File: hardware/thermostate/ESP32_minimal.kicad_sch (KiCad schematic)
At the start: 28 parts, among them IC1 L8050QLT1G, IC2 L8050QLT1G, P1 USB_C_Plug_USB2.0, SW1 SW_Push, SW2 SW_Push, U1 ESP32-S3-WROOM-1, U2 LM1117-3.3

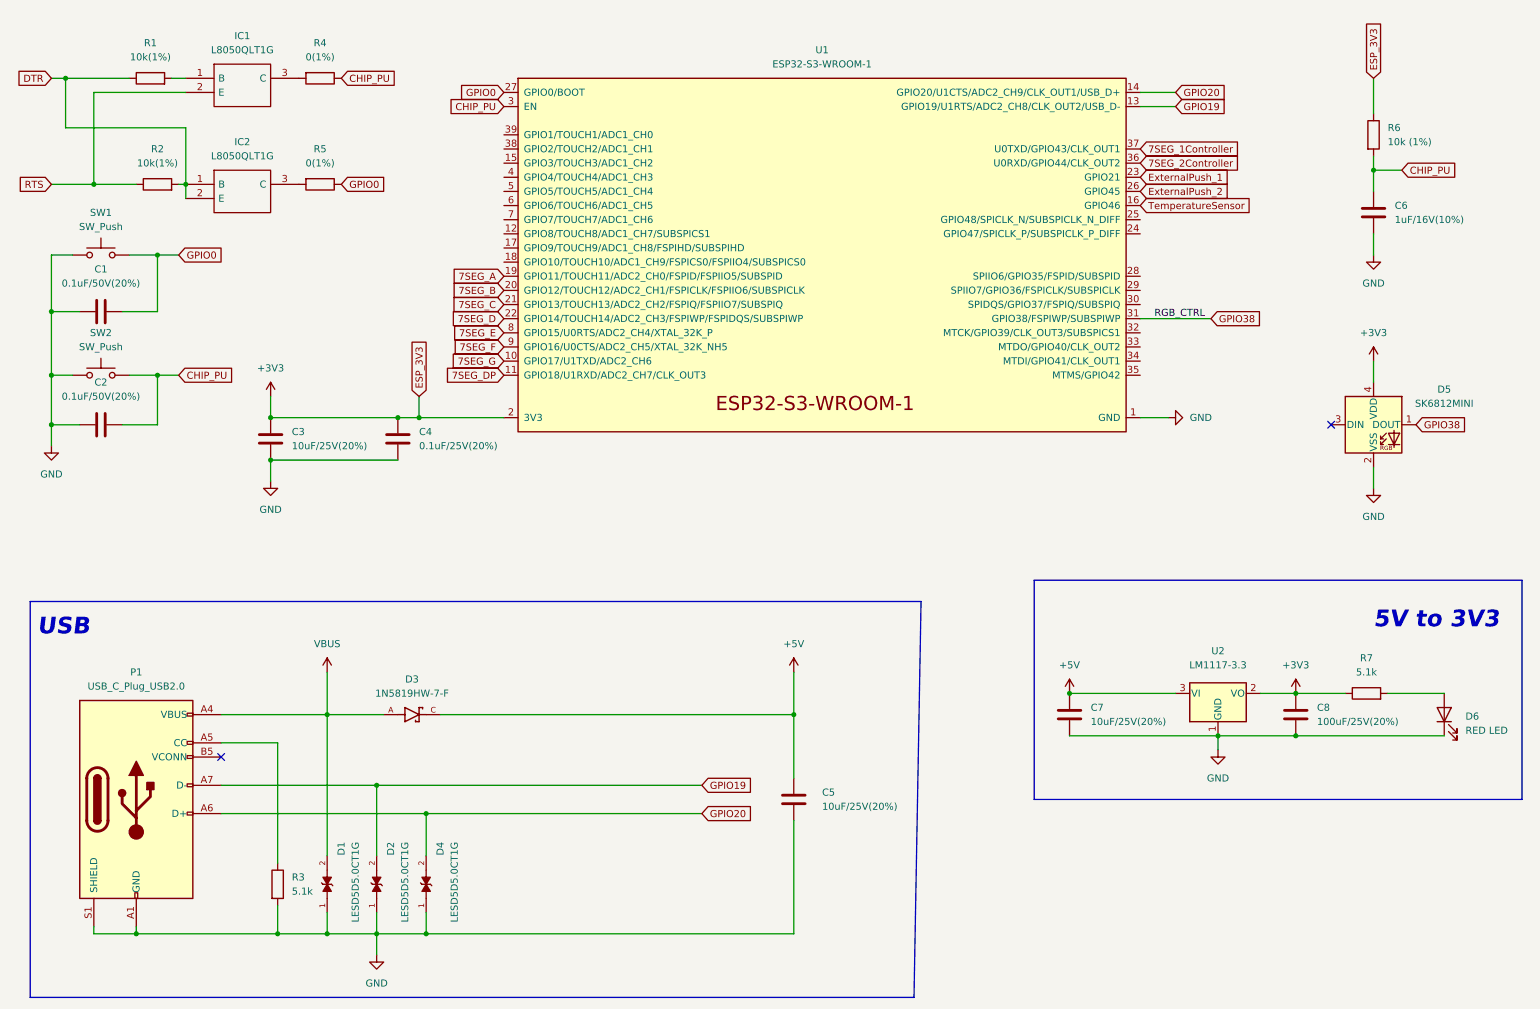
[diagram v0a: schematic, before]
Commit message: Start desing PCB
Signed-off-by: Javier <javierfernandezvillasante@gmail.com>
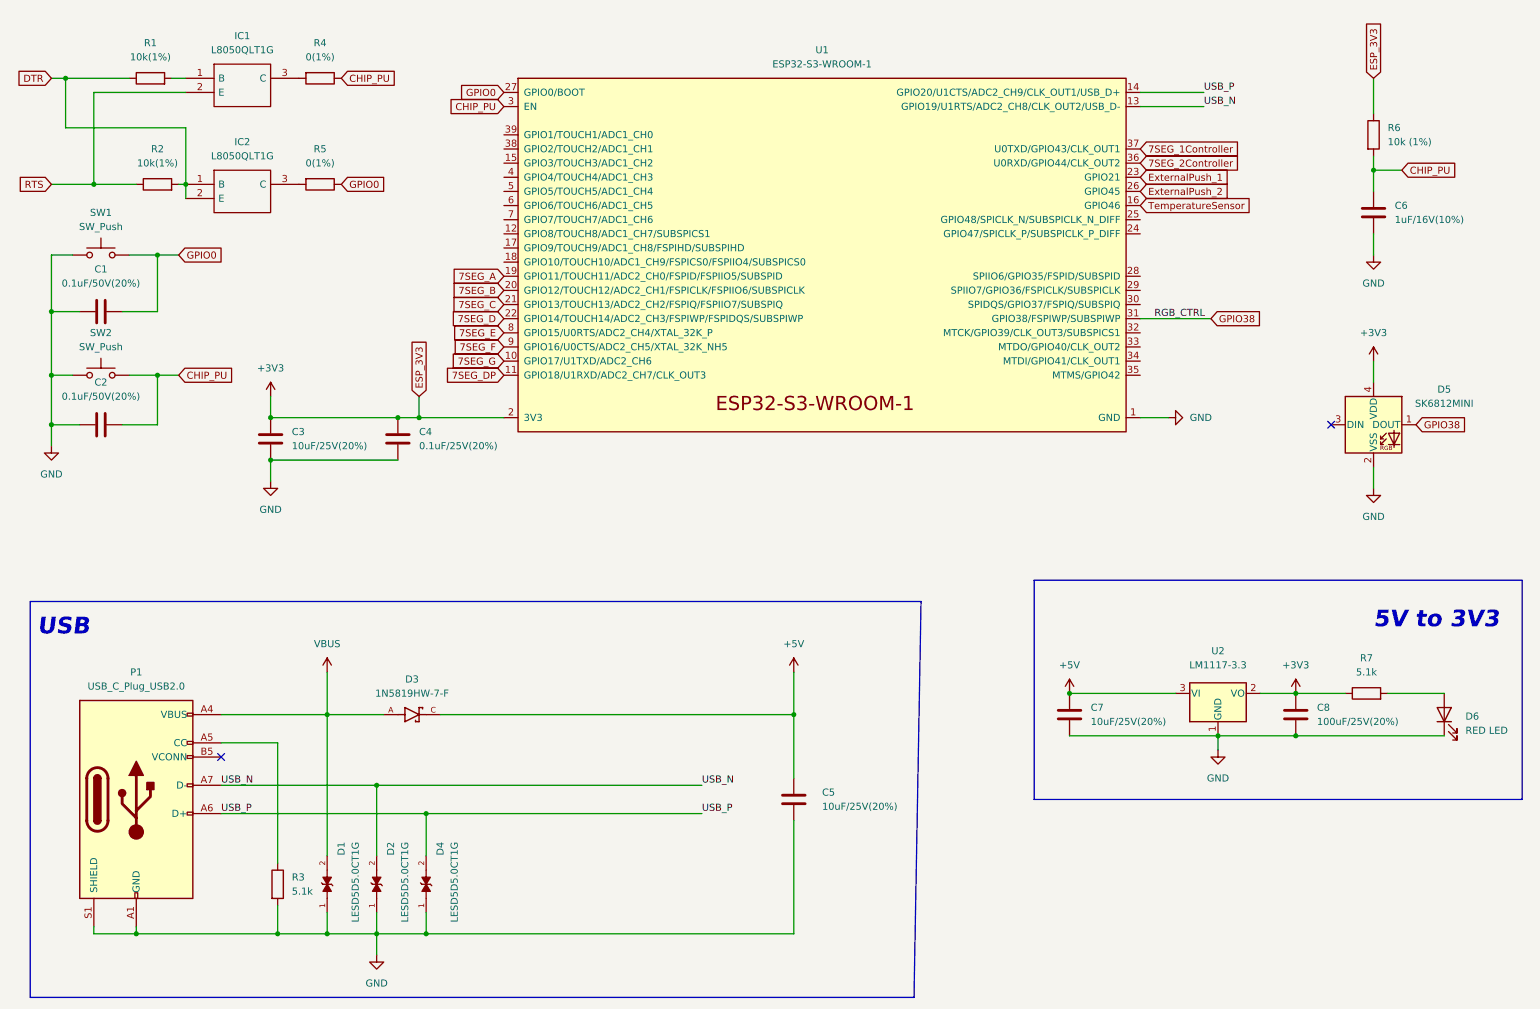
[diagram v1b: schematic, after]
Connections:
- net GPIO19 renamed USB_N
- net GPIO20 renamed USB_P
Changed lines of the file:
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@@
+    (stroke (width 0) (type default) (color 0 0 0 0))
+  )
+  (wire (pts (xy 214.63 33.02) (xy 226.06 33.02))
     (stroke (width 0) (type default) (color 0 0 0 0))
   )
@@
     (stroke (width 0) (type default) (color 0 0 0 0))
   )
-  (wire (pts (xy 220.98 33.02) (xy 214.63 33.02))
-    (stroke (width 0) (type default) (color 0 0 0 0))
-  )
   (wire (pts (xy 21.59 39.37) (xy 21.59 30.48))
     (stroke (width 0) (type default) (color 0 0 0 0))
@@
     (stroke (width 0) (type default) (color 0 0 0 0))
   )
-  (wire (pts (xy 220.98 35.56) (xy 214.63 35.56))
+  (wire (pts (xy 214.63 35.56) (xy 226.06 35.56))
     (stroke (width 0) (type default) (color 0 0 0 0))
   )
@@
     (effects (font (size 3 3) bold italic) (justify left bottom))
   )
+  (label "USB_P" (at 49.53 162.56 0)
+    (effects (font (size 1.27 1.27)) (justify left bottom))
+  )
   (label "RGB_CTRL" (at 217.17 73.66 0)
     (effects (font (size 1.27 1.27)) (justify left bottom))
   )
+  (label "USB_N" (at 226.06 35.56 0)
+    (effects (font (size 1.27 1.27)) (justify left bottom))
+  )
+  (label "USB_N" (at 49.53 157.48 0)
+    (effects (font (size 1.27 1.27)) (justify left bottom))
+  )
+  (label "USB_P" (at 135.89 162.56 0)
+    (effects (font (size 1.27 1.27)) (justify left bottom))
+  )
+  (label "USB_P" (at 226.06 33.02 0)
+    (effects (font (size 1.27 1.27)) (justify left bottom))
+  )
+  (label "USB_N" (at 135.89 157.48 0)
+    (effects (font (size 1.27 1.27)) (justify left bottom))
+  )
   (global_label "GPIO0" (shape input) (at 41.91 62.23 0) (fields_autoplaced)
     (effects (font (size 1.27 1.27)) (justify left))
@@
     )
   )
-  (global_label "GPIO19" (shape input) (at 135.89 157.48 0) (fields_autoplaced)
-    (effects (font (size 1.27 1.27)) (justify left))
-    (property "Intersheet References" "${INTERSHEET_REFS}" (id 0) (at 145.1974 157.4006 0)
-      (effects (font (size 1.27 1.27)) (justify left) hide)
-    )
-  )
   (global_label "ESP_3V3" (shape input) (at 85.09 87.63 90) (fields_autoplaced)
     (effects (font (size 1.27 1.27)) (justify left))
@@
       (effects (font (size 1.27 1.27)) (justify left) hide)
     )
-  )
-  (global_label "GPIO20" (shape input) (at 135.89 162.56 0) (fields_autoplaced)
-    (effects (font (size 1.27 1.27)) (justify left))
-    (property "Intersheet References" "${INTERSHEET_REFS}" (id 0) (at 145.1974 162.4806 0)
-      (effects (font (size 1.27 1.27)) (justify left) hide)
-    )
-  )
-  (global_label "GPIO20" (shape input) (at 220.98 33.02 0) (fields_autoplaced)
-    (effects (font (size 1.27 1.27)) (justify left))
-    (property "Intersheet References" "${INTERSHEET_REFS}" (id 0) (at 230.2874 32.9406 0)
-      (effects (font (size 1.27 1.27)) (justify left) hide)
-    )
-  )
-  (global_label "GPIO19" (shape input) (at 220.98 35.56 0) (fields_autoplaced)
-    (effects (font (size 1.27 1.27)) (justify left))
-    (property "Intersheet References" "${INTERSHEET_REFS}" (id 0) (at 230.2874 35.4806 0)
-      (effects (font (size 1.27 1.27)) (justify left) hide)
-    )
